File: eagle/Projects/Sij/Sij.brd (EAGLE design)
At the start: 100 x 80 mm, 127 parts, among them U1 ATMEGA2560AU, U2 BQ76925_PW_20, U3 LM1085_KTT_3, U4 LM7805, U5 TC7SU04F

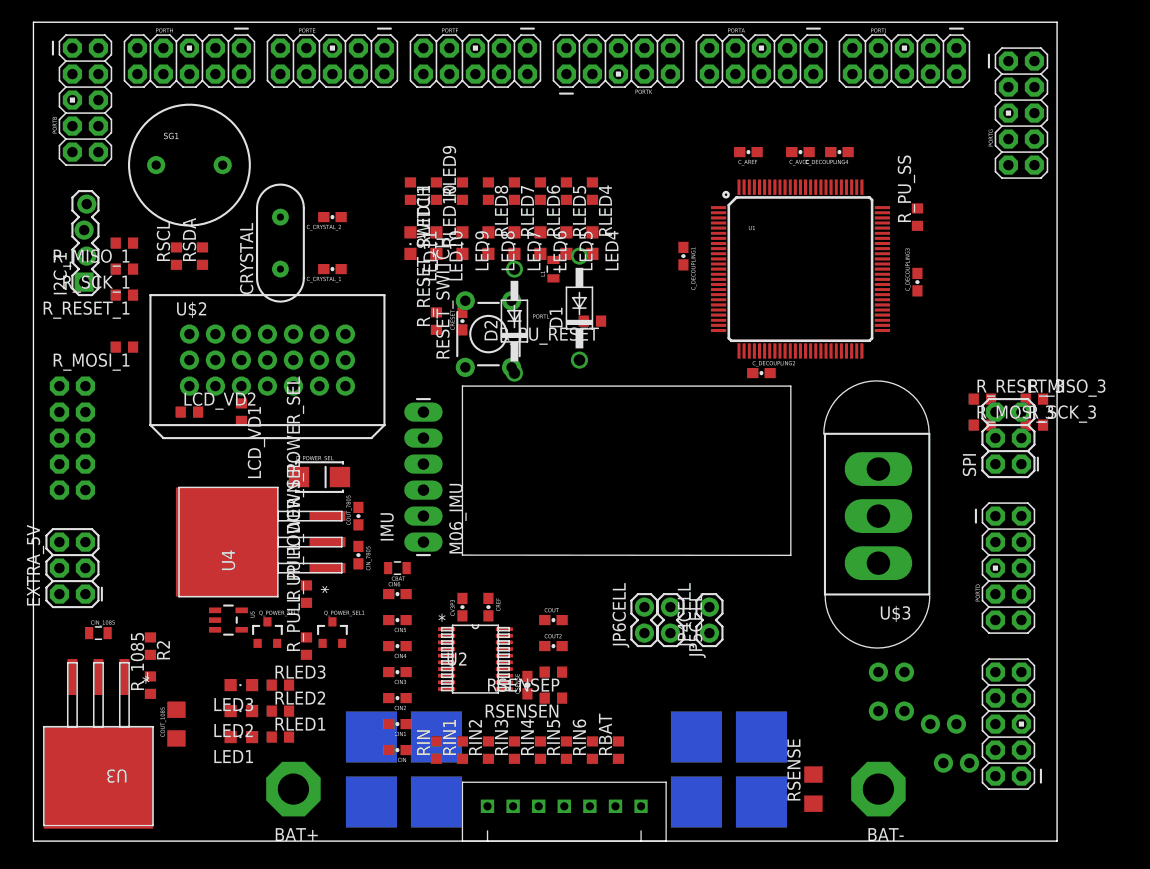
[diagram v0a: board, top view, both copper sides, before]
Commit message: presque terminé le layout. Après genre 20h de travail acharné!
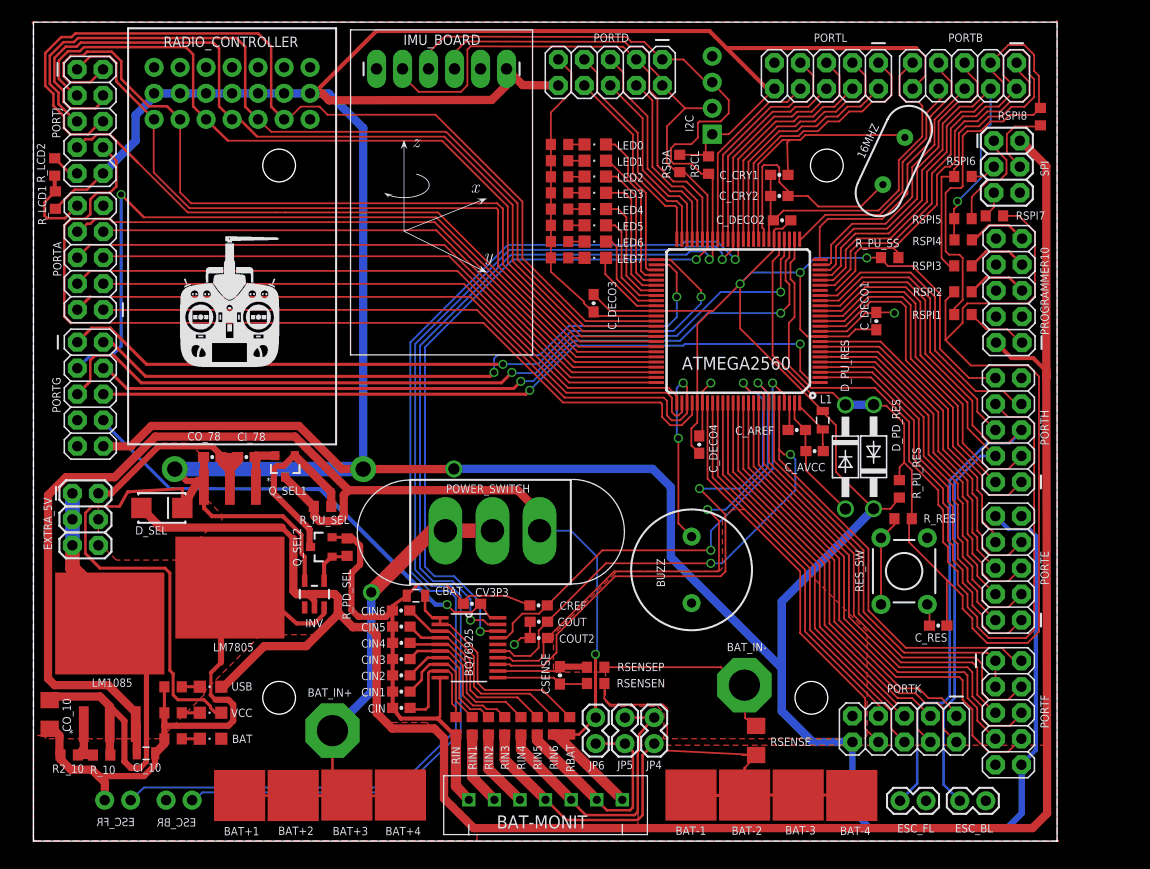
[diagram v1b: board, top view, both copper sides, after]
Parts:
- removed BAT+, BAT-: AWG_10_HOLE_PAD, custom_parts:AWG10_HOLE_PAD
- removed CIN_1085: 10uF, SparkFun-Capacitors:0805
- removed CIN_7805: 0.22uF, SparkFun-Capacitors:0603-CAP
- removed COUT_1085: 10uF, SparkFun-Capacitors:1206
- removed COUT_7805, CRESET, C_DECOUPLING1, C_DECOUPLING2, C_DECOUPLING3, C_DECOUPLING4: 0.1uF, SparkFun-Capacitors:0603-CAP
- removed CRYSTAL: 16MHz, SparkFun-FreqCtrl:HC49US
- removed C_CRYSTAL_1, C_CRYSTAL_2: 20pF, SparkFun-Capacitors:0603-CAP
- removed D1, D2: 1N4004, diode:DO41-10
- removed D_POWER_SEL: CDBA320L, SparkFun-DiscreteSemi:SMA-DIODE_ALT
- removed ESC_BL+, ESC_BL-, ESC_BR+, ESC_BR-, ESC_FL+, ESC_FL-, ESC_FR+, ESC_FR-: BULLET_PAD, custom_parts:4.5MM_SQUARE
- removed ESC_BL_PWM, ESC_BR_PWM, ESC_FL_PWM, ESC_FR_PWM: 640455 TE connectivity, SparkFun-Connectors:1X02
- removed I2C_1: (no value), SparkFun-Connectors:1X04_LOCK
- removed IMU: M06_IMU, custom_parts:1X06_LONGPADS
- removed JP4CELL, JP5CELL, JP6CELL: (no value), SparkFun-Retired:1X02
- removed LCD_VD1, LCD_VD2: (no value), resistor:R0603
- removed LED10, LED11, LED8, LED9: (no value), led:CHIPLED_0805
- removed Q_POWER_SEL1: MOSFET-PCHANNEL, SparkFun-DiscreteSemi:SOT23-3
- removed Q_POWER_SEL2: MOSFET-NCHANNELAO3404A, SparkFun-DiscreteSemi:SOT23-3
- removed R2: adj, resistor:R0603
- removed RESET_SWITCH: SWITCH-MOMENTARY-2PTH, SparkFun-Electromechanical:TACTILE-PTH
- removed RLED10, RLED11, RLED8, RLED9: 91, resistor:R0603
- removed R_1085: 121, resistor:R0603
- removed R_MISO_1, R_MISO_3, R_MOSI_1, R_MOSI_3, R_RESET_1, R_RESET_3, R_SCK_1, R_SCK_3: 500, resistor:R0603
- removed R_PULL_DOWN_POWER_SEL, R_PULL_UP_POWER_SEL: 10K, resistor:R0603
- removed R_PU_RESET: 4.7k, resistor:R0603
- removed R_RESET_SWITCH: 363, resistor:R0603
- removed SG1: BUZZERPTH, SparkFun-Electromechanical:BUZZER-12MM
- removed U$1: 7_PIN_JST-XH, JST-XH_HEADERS:7_PIN_JST-XH
- removed U$2: RF_CONTROL_3X7_CON, custom_parts:3X07
- removed U$3: SWITCH_3_PIN, custom_parts:SWITCH-SPDT_KIT
- removed U1: ATMEGA2560AU, SparkFun-DigitalIC:TQFP100
- removed U2: BQ76925_PW_20, TI:PW20
- removed U3: LM1085_KTT_3, TI:KTT3
- removed U4: LM7805, TI:KTT3
- removed U5: TC7SU04F, SparkFun-DigitalIC:SOT23-5
- added 16MHZ: 16MHz, SparkFun-FreqCtrl:HC49US
- added ATMEGA2560: ATMEGA2560AU, SparkFun-DigitalIC:TQFP100
- added BAT, LED0, USB, VCC: (no value), led:CHIPLED_0805
- added BAT+1, BAT+2, BAT+3, BAT+4, BAT-1, BAT-2, BAT-3, BAT-4: BULLET_PAD, custom_parts:4.5MM_SQUARE
- added BAT-MONIT: 7_PIN_JST-XH, JST-XH_HEADERS:7_PIN_JST-XH
- added BAT_IN+, BAT_IN-: AWG_10_HOLE_PAD, custom_parts:AWG10_HOLE_PAD
- added BQ76925: BQ76925_PW_20, TI:PW20
- added BUZZ: BUZZERPTH, SparkFun-Electromechanical:BUZZER-12MM
- added CI_10: 10uF, SparkFun-Capacitors:0805
- added CI_78: 0.22uF, SparkFun-Capacitors:0603-CAP
- added CO_10: 10uF, SparkFun-Capacitors:1206
- added CO_78, C_DECO1, C_DECO2, C_DECO3, C_DECO4, C_RES: 0.1uF, SparkFun-Capacitors:0603-CAP
- added C_CRY1, C_CRY2: 22pF, SparkFun-Capacitors:0603-CAP
- added D_PD_RES, D_PU_RES: 1N4004, diode:DO41-10
- added D_SEL: CDBA320L, SparkFun-DiscreteSemi:SMA-DIODE_ALT
- added ESC_BL, ESC_BR, ESC_FL, ESC_FR: 640455 TE connectivity, SparkFun-Connectors:1X02
- added I2C: (no value), SparkFun-Connectors:1X04_NO_SILK
- added IMU_BOARD: M06_IMU, custom_parts:1X06_LONGPADS
- added INV: TC7SU04F, SparkFun-DigitalIC:SOT23-5
- added JP4, JP5, JP6: (no value), SparkFun-Retired:1X02
- added LM1085: LM1085_KTT_3, TI:KTT3
- added LM7805: LM7805, TI:KTT3
- added POWER_SWITCH: SWITCH_3_PIN, custom_parts:SWITCH-SPDT_KIT
- added Q_SEL1: MOSFET-PCHANNEL, SparkFun-DiscreteSemi:SOT23-3
- added Q_SEL2: MOSFET-NCHANNELAO3404A, SparkFun-DiscreteSemi:SOT23-3
- added R2_10: adj, resistor:R0603
- added RADIO_CONTROLLER: RF_CONTROL_3X7_CON, custom_parts:3X07
- added RES_SW: SWITCH-MOMENTARY-2PTH, SparkFun-Electromechanical:TACTILE-PTH
- added RLED0, R_BAT, R_USB, R_VCC: (no value), resistor:R0603
- added RSPI1, RSPI2, RSPI3, RSPI4, RSPI5, RSPI6, RSPI7, RSPI8: 500, resistor:R0603
- added R_10: 121, resistor:R0603
- added R_LCD1: 2k, resistor:R0603
- added R_LCD2: 330, resistor:R0603
- added R_PD_SEL, R_PU_SEL: 10K, resistor:R0603
- added R_PU_RES: 4.7k, resistor:R0603
- added R_RES: 363, resistor:R0603
- RLED1, RLED3, RLED4, RLED5, RLED6, RLED7: value 56 -> (none)
- RLED2: value 316 -> (none)
- moved PORTG 95.0 mm to (5.56, 43.7)
- moved PROGRAMMER10 92.6 mm to (95.3, 53.8), flipped to the top
- moved PORTH 87.8 mm to (95.2, 40.2), turned to 180 degrees
- moved PORTB 85.9 mm to (91.0, 74.8), turned to 270 degrees
- moved PORTE 82.6 mm to (95.2, 26.7), turned to 180 degrees
- moved PORTF 82.2 mm to (95.2, 12.5), turned to 0 degrees
- moved PORTJ 79.8 mm to (5.53, 70.3), turned to 0 degrees
- moved PORTK 71.0 mm to (85.1, 11.0), turned to 270 degrees
- moved PORTA 68.3 mm to (5.56, 57.0), turned to 180 degrees
- moved LED1 66.1 mm to (54.9, 66.5)
- moved PORTL 65.8 mm to (77.5, 74.8), turned to 270 degrees
- moved LED2 62.6 mm to (54.9, 64.9)
- moved RLED1 62.6 mm to (51.4, 66.5), turned to 180 degrees
- moved PORTD 62.1 mm to (56.4, 75.1), turned to 270 degrees
- moved LED3 59.2 mm to (54.9, 63.3)
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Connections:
- removed net N$49: RLED6.1, U1.58
- removed net N$50: RLED7.1, U1.57
- removed net N$51: RLED8.1, U1.56
- removed net N$52: RLED9.1, U1.55
- removed net N$53: RLED10.1, U1.54
- removed net N$54: RLED11.1, U1.53
- removed net PB0: PORTB.1
- removed net PB1: PORTB.2
- removed net PB2: PORTB.3
- removed net PB3: PORTB.4
- removed net PD0: PORTD.1
- removed net PD1: PORTD.2
- removed net PD2: PORTD.3
- removed net PF0: PORTF.1
- removed net PF0_PF2: CREF.1, U1.95, U1.97, U2.17
- removed net PF2: PORTF.3
- removed net RLED2: LED2.A, RLED2.2
- new net N$14: ATMEGA2560.60, LED7.A
- new net N$20: ATMEGA2560.58, LED5.A
- new net N$21: ATMEGA2560.57, LED4.A
- new net N$22: ATMEGA2560.56, LED3.A
- new net N$31: ATMEGA2560.53, LED0.A
- new net N$40: LED6.C, RLED6.1
- new net PF0_2: ATMEGA2560.95, ATMEGA2560.97, BQ76925.17, CREF.1, PORTF.1, PORTF.3
- net BAT+: now also BAT+1.IN, BAT+2.IN, BAT+3.IN, BAT+4.IN, BAT.A, BAT_IN+.BAT_CONNECTOR, POWER_SWITCH.2, POWER_SWITCH.3; no longer BAT+.BAT_CONNECTOR, ESC_BL+.IN, ESC_BR+.IN, ESC_FL+.IN, ESC_FR+.IN, RLED2.1, U$3.2, U$3.3
- net BAT-: now also BAT_IN-.BAT_CONNECTOR; no longer BAT-.BAT_CONNECTOR
- net CH1: now also ATMEGA2560.68, RADIO_CONTROLLER.15; no longer U$2.15, U1.63
- net CH2: now also ATMEGA2560.67, RADIO_CONTROLLER.16; no longer U$2.16, U1.64
- net CH3: now also ATMEGA2560.66, RADIO_CONTROLLER.17; no longer U$2.17, U1.65
- net CH4: now also ATMEGA2560.65, RADIO_CONTROLLER.18; no longer U$2.18, U1.66
- net CH5: now also ATMEGA2560.64, RADIO_CONTROLLER.19; no longer U$2.19, U1.67
- net CH6: now also ATMEGA2560.63, RADIO_CONTROLLER.20; no longer U$2.20, U1.68
- net CV3P3: now also BQ76925.20, CV3P3.1
- net GND: now also ATMEGA2560.11, ATMEGA2560.32, ATMEGA2560.62, ATMEGA2560.81, ATMEGA2560.99, BAT-MONIT.P$1, BQ76925.10, BUZZ.+, CI_10.2, CI_78.2, CO_10.2, CO_78.2, C_CRY1.1, C_CRY2.1, C_DECO1.2, C_DECO2.2, C_DECO3.2, C_DECO4.2, C_RES.2, D_PD_RES.A, ESC_BL.2, ESC_BR.2, ESC_FL.2, ESC_FR.2, I2C.4, IMU_BOARD.1, IMU_BOARD.5, INV.3, LM7805.2, LM7805.4, Q_SEL2.2, R2_10.1, RADIO_CONTROLLER.1, RADIO_CONTROLLER.2, RADIO_CONTROLLER.3, RADIO_CONTROLLER.4, RADIO_CONTROLLER.5, RADIO_CONTROLLER.6, RADIO_CONTROLLER.7, RES_SW.3, RES_SW.4, RLED0.2, RLED1.2, RLED2.2, RLED3.2, RLED4.2, RLED5.2, RLED6.2, RLED7.2, R_BAT.2, R_LCD2.1, R_PD_SEL.1, R_USB.2, R_VCC.2; no longer CIN_1085.2, CIN_7805.2, COUT_1085.2, COUT_7805.2, CRESET.2, C_CRYSTAL_1.1, C_CRYSTAL_2.1, C_DECOUPLING1.2, C_DECOUPLING2.2, C_DECOUPLING3.2, C_DECOUPLING4.2, D1.A, ESC_BL_PWM.2, ESC_BR_PWM.2, ESC_FL_PWM.2, ESC_FR_PWM.2, I2C_1.4, IMU.1, IMU.5, LCD_VD2.1, LED1.C, LED10.C, LED11.C, LED2.C, LED3.C, LED4.C, LED5.C, LED6.C, LED7.C, LED8.C, LED9.C, Q_POWER_SEL2.2, R2.1, RESET_SWITCH.3, R_PULL_DOWN_POWER_SEL.1, SG1.+, U$1.P$1, U$2.1, U$2.2, U$2.3, U$2.4, U$2.5, U$2.6, U$2.7, U1.11, U1.32, U1.62, U1.81, U1.99, U2.10, U4.2, U4.4, U5.3
- net GND-ISO: now also BAT-1.IN, BAT-2.IN, BAT-3.IN, BAT-4.IN; no longer ESC_BL-.IN, ESC_BR-.IN, ESC_FL-.IN, ESC_FR-.IN
- net INT_IMU: now also ATMEGA2560.45, IMU_BOARD.2, PORTD.3; no longer IMU.2, U1.45
- net LCD_V0: now also R_LCD1.1, R_LCD2.2; no longer LCD_VD1.1, LCD_VD2.2
- net MISO: now also ATMEGA2560.22, PORTB.4, RSPI4.1, RSPI5.1; no longer R_MISO_1.1, R_MISO_3.1, U1.22
- net MOSI: now also ATMEGA2560.21, PORTB.3, RSPI1.1, RSPI8.1; no longer R_MOSI_1.1, R_MOSI_3.1, U1.21
- net N$1: now also RSPI3.2; no longer R_SCK_1.2
- net N$10: now also BQ76925.8; no longer U2.8
- net N$11: now also BQ76925.9; no longer U2.9
- net N$12: now also BQ76925.5; no longer U2.5
- net N$13: now also INV.4, Q_SEL2.1, R_PD_SEL.2; no longer Q_POWER_SEL2.1, R_PULL_DOWN_POWER_SEL.2, U5.4
- net N$15: now also BQ76925.11; no longer U2.11
- net N$16: now also BQ76925.12; no longer U2.12
- net N$17: now also BQ76925.3; no longer U2.3
- net N$18: now also BQ76925.4; no longer U2.4
- net N$19: now also ATMEGA2560.59, LED6.A; no longer LED4.A, RLED4.2
- net N$2: now also RSPI1.2; no longer R_MOSI_1.2
- net N$23: now also BAT-MONIT.P$2; no longer U$1.P$2
- net N$24: now also RSPI8.2; no longer R_MOSI_3.2
- net N$25: now also ATMEGA2560.55, LED2.A; no longer LED5.A, RLED5.2
- net N$26: now also ATMEGA2560.54, LED1.A; no longer CV3P3.1, U2.20
- net N$27: now also BAT-MONIT.P$3; no longer U$1.P$3
- net N$28: now also BAT-MONIT.P$4, JP4.1; no longer JP4CELL.1, U$1.P$4
- net N$29: now also BAT-MONIT.P$5, JP4.2, JP5.1; no longer JP4CELL.2, JP5CELL.1, U$1.P$5
- net N$3: now also RSPI4.2; no longer R_MISO_1.2
- net N$30: now also BAT-MONIT.P$6, JP5.2, JP6.1; no longer JP5CELL.2, JP6CELL.1, U$1.P$6
- net N$32: now also CO_10.1, LM1085.2, LM1085.4, R_10.1; no longer COUT_1085.1, R_1085.1, U3.2, U3.4
- net N$33: now also LM1085.1, R2_10.2, R_10.2; no longer R2.2, R_1085.2, U3.1
- net N$34: now also RES_SW.1, RES_SW.2, R_RES.2; no longer RESET_SWITCH.1, R_RESET_SWITCH.2
- net N$35: now also R_USB.1, USB.C; no longer LED1.A, RLED1.2
- net N$36: now also 16MHZ.2, ATMEGA2560.33, C_CRY2.2; no longer CRYSTAL.2, C_CRYSTAL_2.2, U1.33
- net N$37: now also Q_SEL1.1, Q_SEL2.3, R_PU_SEL.1; no longer Q_POWER_SEL1.1, Q_POWER_SEL2.3, R_PULL_UP_POWER_SEL.1
- net N$38: now also R_VCC.1, VCC.C; no longer LED3.A, RLED3.2
- net N$39: now also LED7.C, RLED7.1; no longer LED6.A, RLED6.2
- net N$4: now also CI_78.1, LM7805.1, Q_SEL1.2; no longer CIN_7805.1, Q_POWER_SEL1.2, U4.1
- net N$41: now also LED5.C, RLED5.1; no longer LED7.A, RLED7.2
- net N$42: now also RSPI6.2; no longer R_SCK_3.2
- net N$43: now also LED4.C, RLED4.1; no longer LED8.A, RLED8.2
- net N$44: now also LED3.C, RLED3.1; no longer LED9.A, RLED9.2
- net N$45: now also LED2.C, RLED2.1; no longer LED10.A, RLED10.2
- net N$46: now also LED1.C, RLED1.1; no longer LED11.A, RLED11.2
- net N$47: now also LED0.C, RLED0.1; no longer RLED4.1, U1.60
- net N$48: now also BAT.C, R_BAT.1; no longer RLED5.1, U1.59
- net N$5: now also ATMEGA2560.100; no longer U1.100
- net N$55: now also RSPI5.2; no longer R_MISO_3.2
- net N$6: now also 16MHZ.1, ATMEGA2560.34, C_CRY1.2; no longer CRYSTAL.1, C_CRYSTAL_1.2, U1.34
- net N$61: now also RSPI2.2; no longer R_RESET_1.2
- net N$62: now also ATMEGA2560.98; no longer U1.98
- net N$64: now also RSPI7.2; no longer R_RESET_3.2
- net N$7: now also BQ76925.6; no longer U2.6
- net N$8: now also BQ76925.1, BQ76925.2; no longer U2.1, U2.2
- net N$9: now also BQ76925.7; no longer U2.7
- net PA0: now also ATMEGA2560.78, BUZZ.-; no longer SG1.-, U1.78
- net PA1: now also ATMEGA2560.77; no longer U1.77
- net PA2: now also ATMEGA2560.76; no longer U1.76
- net PA3: now also ATMEGA2560.75; no longer PORTD.4, U1.75
- net PA4: now also ATMEGA2560.74; no longer U1.74
- net PA5: now also ATMEGA2560.73; no longer U1.73
- net PA6: now also ATMEGA2560.72; no longer U1.72
- net PA7: now also ATMEGA2560.71; no longer U1.71
- net PB4: now also ATMEGA2560.23; no longer U1.23
- net PB5: now also ATMEGA2560.24; no longer U1.24
- net PB6: now also ATMEGA2560.25; no longer U1.25
- net PB7: now also ATMEGA2560.26; no longer U1.26
- net PD3: now also ATMEGA2560.46, PORTD.4; no longer U1.46
- net PD4: now also ATMEGA2560.47; no longer U1.47
- net PD5: now also ATMEGA2560.48; no longer U1.48
- net PD6: now also ATMEGA2560.49; no longer U1.49
- net PD7: now also ATMEGA2560.50; no longer U1.50
- net PE0: now also ATMEGA2560.2; no longer U1.2
- net PE1: now also ATMEGA2560.3; no longer U1.3
- net PE2: now also ATMEGA2560.4; no longer U1.4
- net PE3: now also ATMEGA2560.5; no longer U1.5
- net PE4: now also ATMEGA2560.6; no longer U1.6
- net PE5: now also ATMEGA2560.7; no longer U1.7
- net PE6: now also ATMEGA2560.8; no longer U1.8
- net PE7: now also ATMEGA2560.9; no longer U1.9
- net PF1: now also ATMEGA2560.96, BQ76925.15; no longer U1.96, U2.15
- net PF3: now also ATMEGA2560.94, BQ76925.14; no longer U1.94, U2.14
- net PF4: now also ATMEGA2560.93, BQ76925.13; no longer U1.93, U2.13
- net PF5: now also ATMEGA2560.92; no longer U1.92
- net PF6: now also ATMEGA2560.91; no longer U1.91
- net PF7: now also ATMEGA2560.90; no longer U1.90
- net PG0: now also ATMEGA2560.51; no longer U1.51
- net PG1: now also ATMEGA2560.52; no longer U1.52
- net PG2: now also ATMEGA2560.70; no longer U1.70
- net PG3: now also ATMEGA2560.28; no longer U1.28
- net PG4: now also ATMEGA2560.29; no longer U1.29
- net PG5: now also ATMEGA2560.1; no longer U1.1
- net PH0: now also ATMEGA2560.12; no longer U1.12
- net PH1: now also ATMEGA2560.13; no longer U1.13
- net PH2: now also ATMEGA2560.14; no longer U1.14
- net PH3: now also ATMEGA2560.15, ESC_BL.1; no longer ESC_BL_PWM.1, U1.15
- net PH4: now also ATMEGA2560.16, ESC_FL.1; no longer ESC_FL_PWM.1, U1.16
- net PH5: now also ATMEGA2560.17; no longer U1.17
- net PH6: now also ATMEGA2560.18; no longer U1.18
- net PH7: now also ATMEGA2560.27; no longer U1.27
- net PJ6: now also ATMEGA2560.69; no longer U1.69
- net PJ7: now also ATMEGA2560.79; no longer U1.79
- net PK0: now also ATMEGA2560.89; no longer U1.89
- net PK1: now also ATMEGA2560.88; no longer U1.88
- net PK2: now also ATMEGA2560.87; no longer U1.87
- net PK3: now also ATMEGA2560.86; no longer U1.86
- net PK4: now also ATMEGA2560.85; no longer U1.85
- net PK5: now also ATMEGA2560.84; no longer U1.84
- net PK6: now also ATMEGA2560.83; no longer U1.83
- net PK7: now also ATMEGA2560.82; no longer U1.82
- net PL0: now also ATMEGA2560.35; no longer U1.35
- net PL1: now also ATMEGA2560.36; no longer U1.36
- net PL2: now also ATMEGA2560.37; no longer U1.37
- net PL3: now also ATMEGA2560.38, ESC_FR.1; no longer ESC_FR_PWM.1, U1.38
- net PL4: now also ATMEGA2560.39, ESC_BR.1; no longer ESC_BR_PWM.1, U1.39
- net PL5: now also ATMEGA2560.40; no longer U1.40
- net PL6: now also ATMEGA2560.41; no longer U1.41
- net PL7: now also ATMEGA2560.42; no longer U1.42
- net RESET: now also ATMEGA2560.30, C_RES.1, D_PD_RES.C, D_PU_RES.A, RSPI2.1, RSPI7.1, R_PU_RES.1, R_RES.1; no longer CRESET.1, D1.C, D2.A, R_PU_RESET.1, R_RESET_1.1, R_RESET_3.1, R_RESET_SWITCH.1, U1.30
- net SCK: now also ATMEGA2560.20, PORTB.2, RSPI3.1, RSPI6.1; no longer R_SCK_1.1, R_SCK_3.1, U1.20
- net SCL: now also ATMEGA2560.43, BQ76925.19, I2C.3, IMU_BOARD.3, PORTD.1; no longer I2C_1.3, IMU.3, U1.43, U2.19
- net SDA: now also ATMEGA2560.44, BQ76925.18, I2C.2, IMU_BOARD.4, PORTD.2; no longer I2C_1.2, IMU.4, U1.44, U2.18
- net SS: now also ATMEGA2560.19, PORTB.1; no longer U1.19
- net VCC: now also ATMEGA2560.10, ATMEGA2560.31, ATMEGA2560.61, ATMEGA2560.80, CO_78.1, C_DECO1.1, C_DECO2.1, C_DECO3.1, C_DECO4.1, D_PU_RES.C, D_SEL.C, I2C.1, IMU_BOARD.6, INV.5, LM7805.3, RADIO_CONTROLLER.10, RADIO_CONTROLLER.11, RADIO_CONTROLLER.12, RADIO_CONTROLLER.13, RADIO_CONTROLLER.14, RADIO_CONTROLLER.8, RADIO_CONTROLLER.9, R_LCD1.2, R_PU_RES.2, VCC.A; no longer COUT_7805.1, C_DECOUPLING1.1, C_DECOUPLING2.1, C_DECOUPLING3.1, C_DECOUPLING4.1, D2.C, D_POWER_SEL.C, I2C_1.1, IMU.6, LCD_VD1.2, RLED1.1, R_PU_RESET.2, SPI.2, U$2.10, U$2.11, U$2.12, U$2.13, U$2.14, U$2.8, U$2.9, U1.10, U1.31, U1.61, U1.80, U4.3, U5.5
- net V_BATT: now also BAT-MONIT.P$7, CI_10.1, JP6.2, LM1085.3, POWER_SWITCH.1, Q_SEL1.3, R_PU_SEL.2; no longer CIN_1085.1, JP6CELL.2, Q_POWER_SEL1.3, R_PULL_UP_POWER_SEL.2, U$1.P$7, U$3.1, U3.3
- net V_USB: now also D_SEL.A, INV.2, SPI.2, USB.A; no longer D_POWER_SEL.A, RLED3.1, U5.2
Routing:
- net VCC: track 0.00 -> 561.4 mm, vias 0 -> 6
- net GND: track 0.00 -> 250.2 mm, vias 0 -> 3
- net V_USB: track 0.00 -> 203.2 mm
- net V_BATT: track 0.00 -> 136.6 mm, vias 0 -> 1
- net PL3: track 0.00 -> 135.9 mm, vias 0 -> 1
- net PL4: track 0.00 -> 131.7 mm, vias 0 -> 1
- net RESET: track 0.00 -> 126.2 mm
- net SCL: track 0.00 -> 122.8 mm, vias 0 -> 2
- net SDA: track 0.00 -> 112.0 mm, vias 0 -> 2
- net PF4: track 0.00 -> 100.0 mm, vias 0 -> 2
- net PF3: track 0.00 -> 97.0 mm, vias 0 -> 2
- net CH6: track 0.00 -> 92.5 mm
- net PF0_2: track 0.00 -> 89.3 mm, vias 0 -> 2
- net PJ7: track 0.00 -> 88.8 mm
- net CH4: track 0.00 -> 87.3 mm
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- added copper zone on layer 1, net BAT+
- added copper zone on layer 1, net BAT-
- added copper zone on layer 1, net GND
- added copper zone on layer 16, net GND
- added copper zone on layer 1, net GND-ISO
- added copper zone on layer 1, net VCC
